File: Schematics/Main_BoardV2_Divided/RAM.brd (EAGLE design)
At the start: 167.6 x 178.7 mm, 46 parts

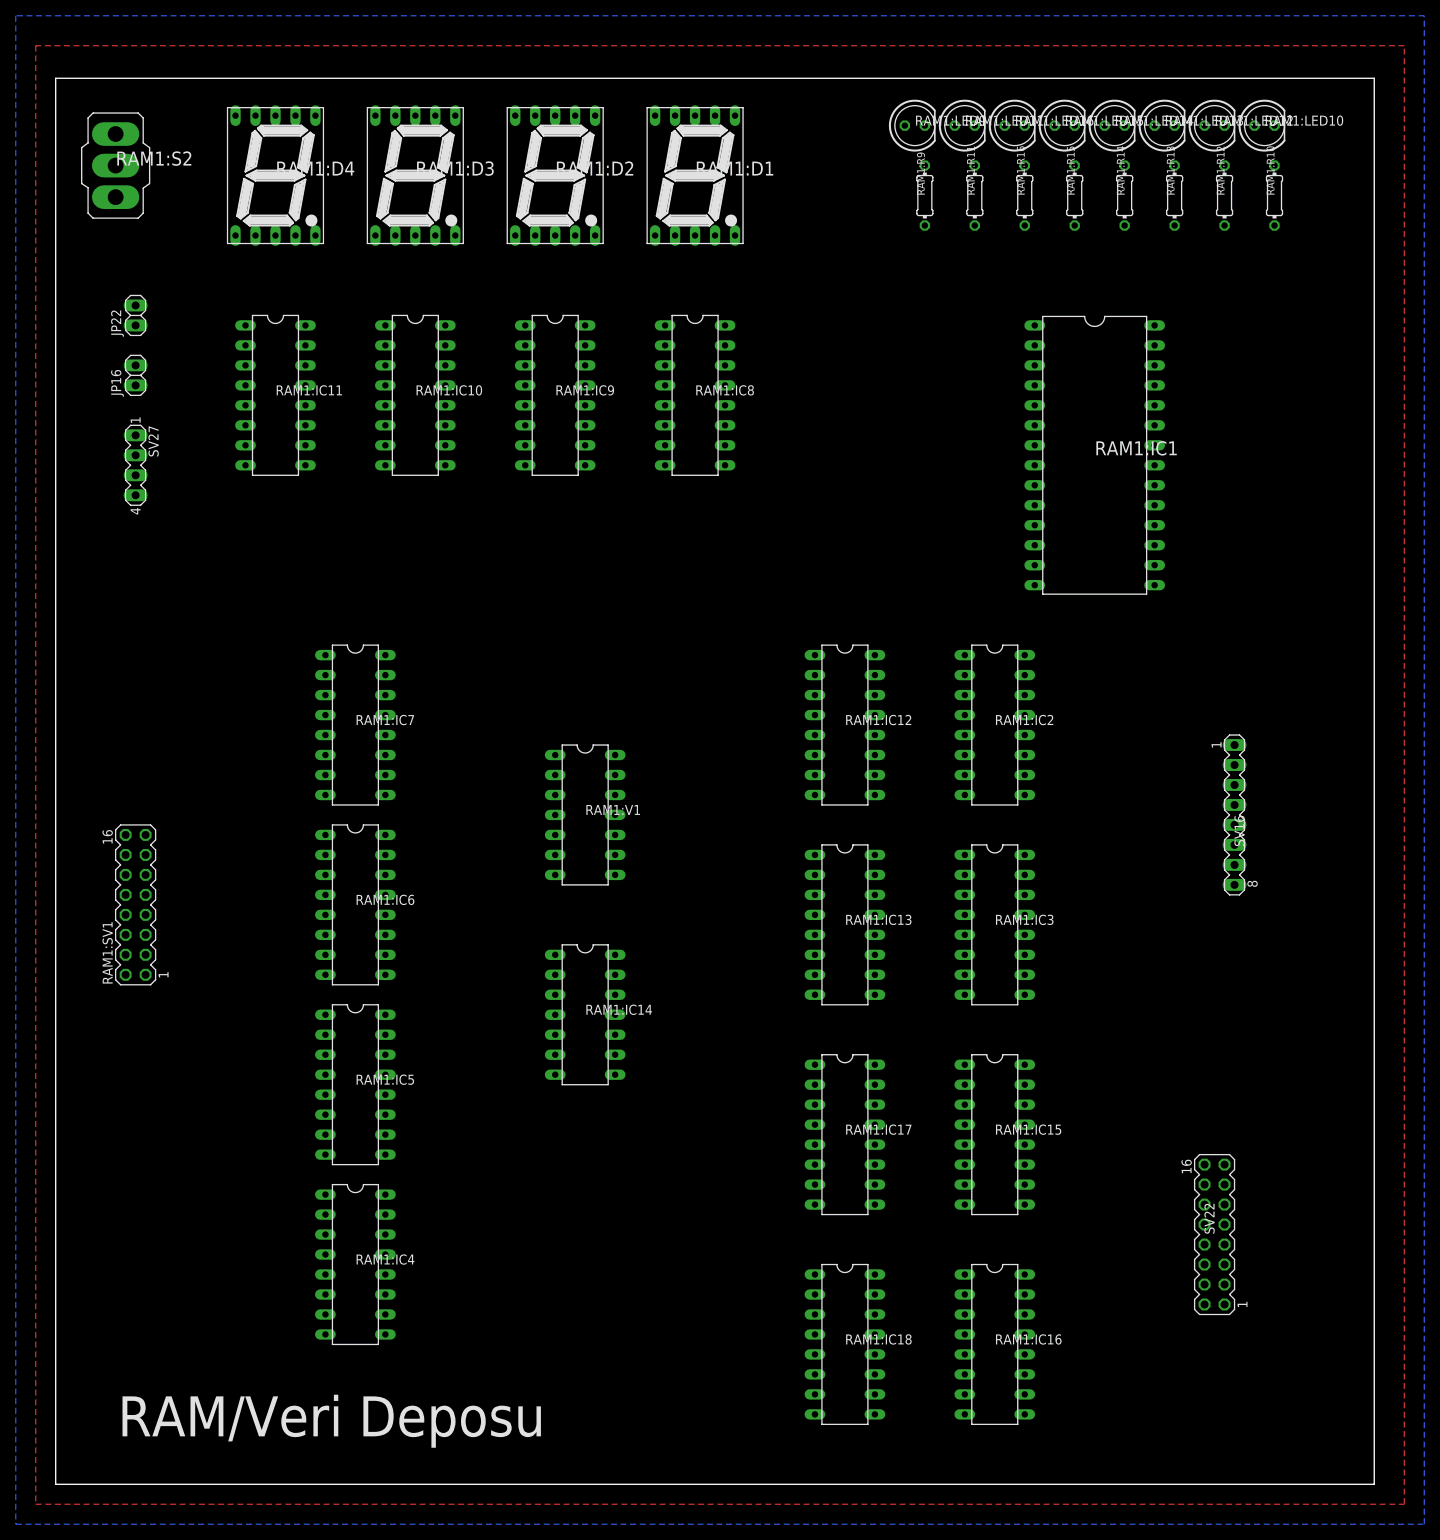
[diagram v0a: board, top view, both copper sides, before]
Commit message: Routd and Cams Created
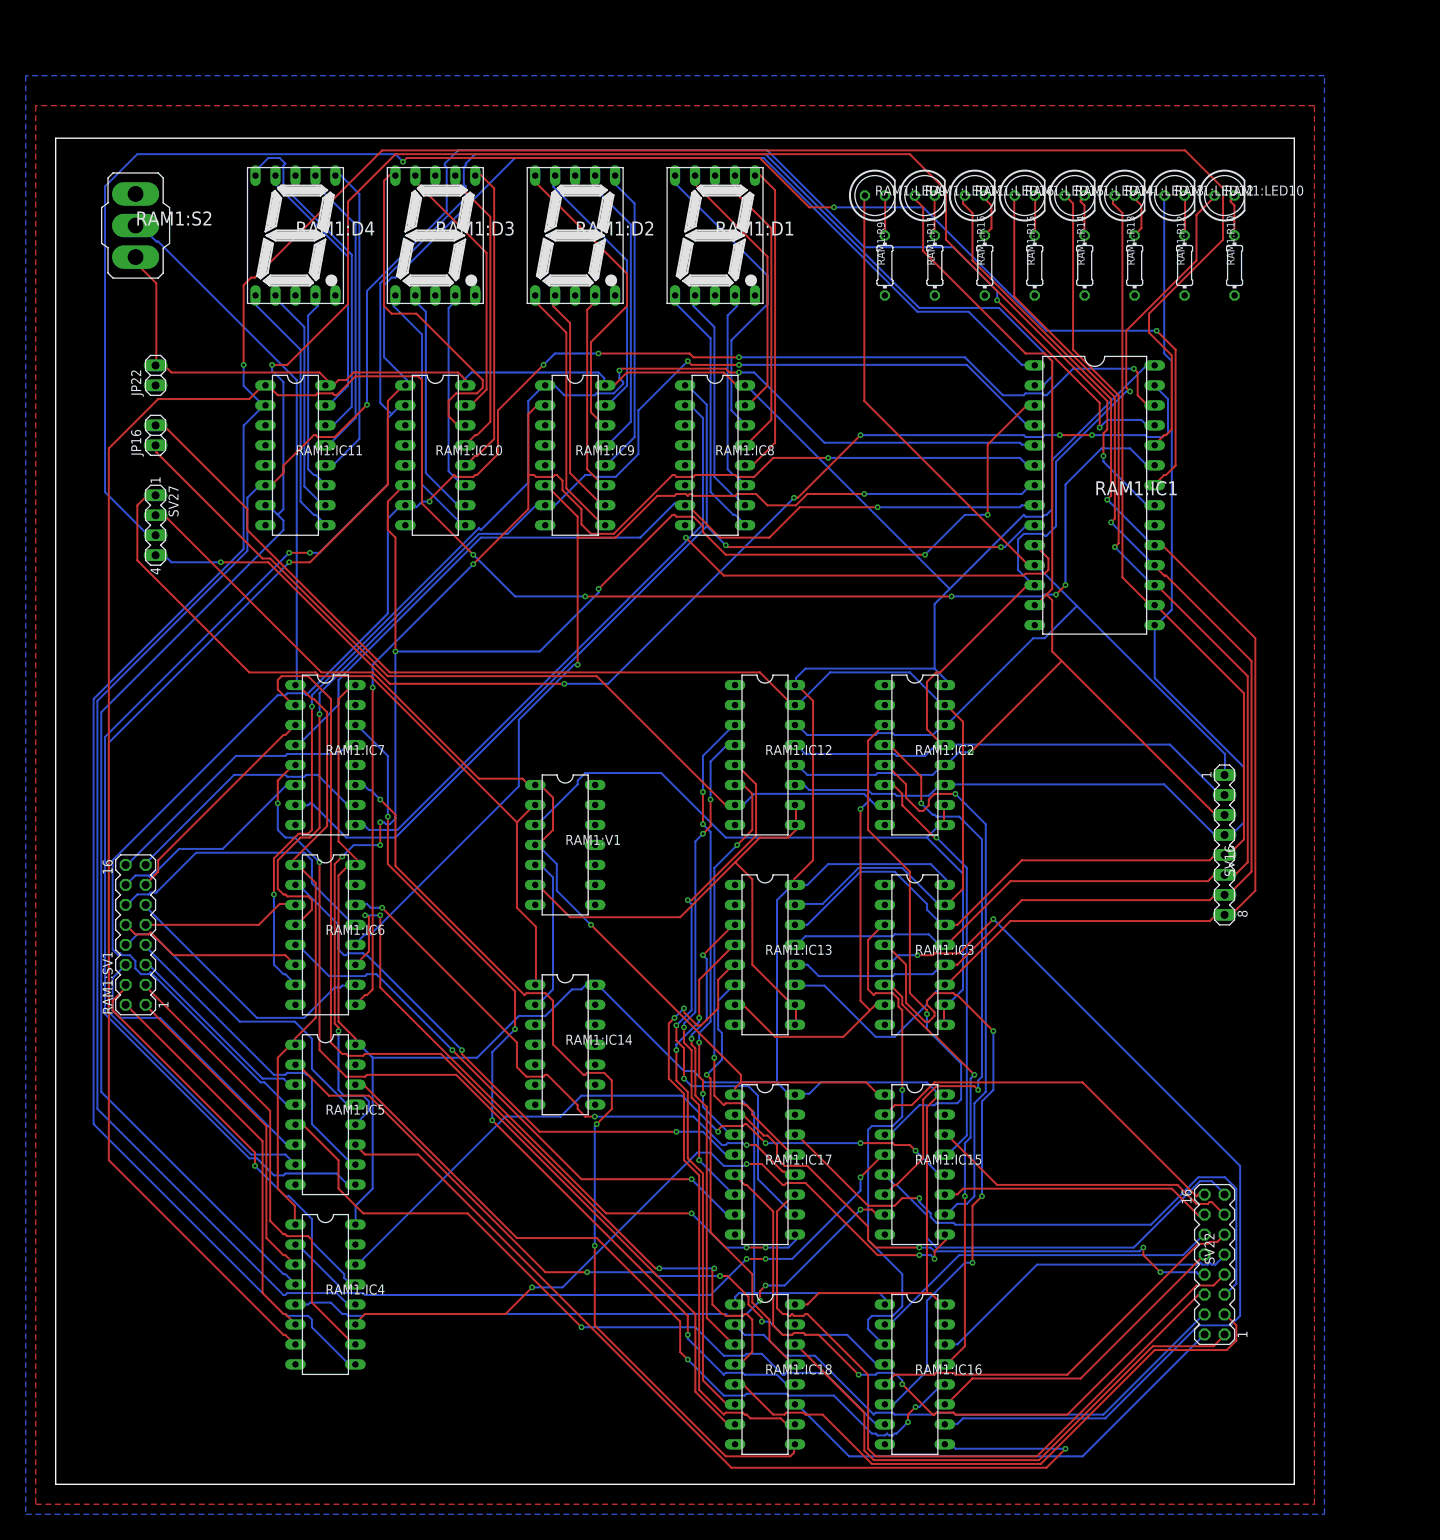
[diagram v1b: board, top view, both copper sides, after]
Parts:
- moved RAM1:IC12 10.9 mm to (90.2, 94.0)
- moved RAM1:IC13 10.9 mm to (90.2, 68.6)
- moved RAM1:IC15 10.9 mm to (109.2, 41.9)
- moved RAM1:IC16 10.9 mm to (109.2, 15.2)
- moved RAM1:IC17 10.9 mm to (90.2, 41.9)
- moved RAM1:IC18 10.9 mm to (90.2, 15.2)
- moved RAM1:IC2 10.9 mm to (109.2, 94.0)
- moved RAM1:IC3 10.9 mm to (109.2, 68.6)
- moved RAM1:LED13 10.2 mm to (135.9, 165.1)
- moved RAM1:LED14 10.2 mm to (129.5, 165.1)
- moved RAM1:LED15 10.2 mm to (123.2, 165.1)
- moved RAM1:LED11 10.2 mm to (110.5, 165.1)
- moved RAM1:LED16 10.2 mm to (116.8, 165.1)
- moved RAM1:LED9 10.2 mm to (104.1, 165.1)
- moved RAM1:LED10 10.2 mm to (148.6, 165.1)
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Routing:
- net VCC: track 0.00 -> 490.5 mm
- net RAM1:N$40: track 0.00 -> 336.2 mm, vias 0 -> 1
- net RAM1:N$37: track 0.00 -> 299.2 mm, vias 0 -> 5
- net RAM1:N$36: track 0.00 -> 298.6 mm, vias 0 -> 2
- net RAM1:N$41: track 0.00 -> 293.4 mm, vias 0 -> 3
- net RAM1:N$44: track 0.00 -> 264.7 mm, vias 0 -> 2
- net RAM1:N$43: track 0.00 -> 243.3 mm, vias 0 -> 1
- net RAM1:N$42: track 0.00 -> 221.4 mm, vias 0 -> 5
- net |RAM_OUT: track 0.00 -> 214.5 mm, vias 0 -> 3
- net RAM1:N$45: track 0.00 -> 197.3 mm, vias 0 -> 8
- net SLC_ADDR: track 0.00 -> 182.7 mm, vias 0 -> 1
- net 8B_8: track 0.00 -> 174.5 mm, vias 0 -> 1
- net CLR: track 0.00 -> 171.0 mm
- net CLK: track 0.00 -> 163.7 mm, vias 0 -> 1
- net 8B_7: track 0.00 -> 163.2 mm, vias 0 -> 1
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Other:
- board size 167.6 x 178.7 mm -> 157.5 x 171.1 mm
- board text added: "16Bit Bus"
- board text added: "8Bit Buffer"
- board text added: "A/M Select"
- board text added: "Address"
- board text added: "Control Signals"
- board text added: "Manual Inputs"
